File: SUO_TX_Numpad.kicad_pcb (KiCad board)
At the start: 2 copper layers, 79.1 x 127.6 mm, 94 parts, among them J1 USB_C_Receptacle_USB2.0_16P, SW1 BOOT, U1 STM32F411CEUx, U2 XC6206PxxxMR-Regulator_Linear, U3 USBLC6-2SC6

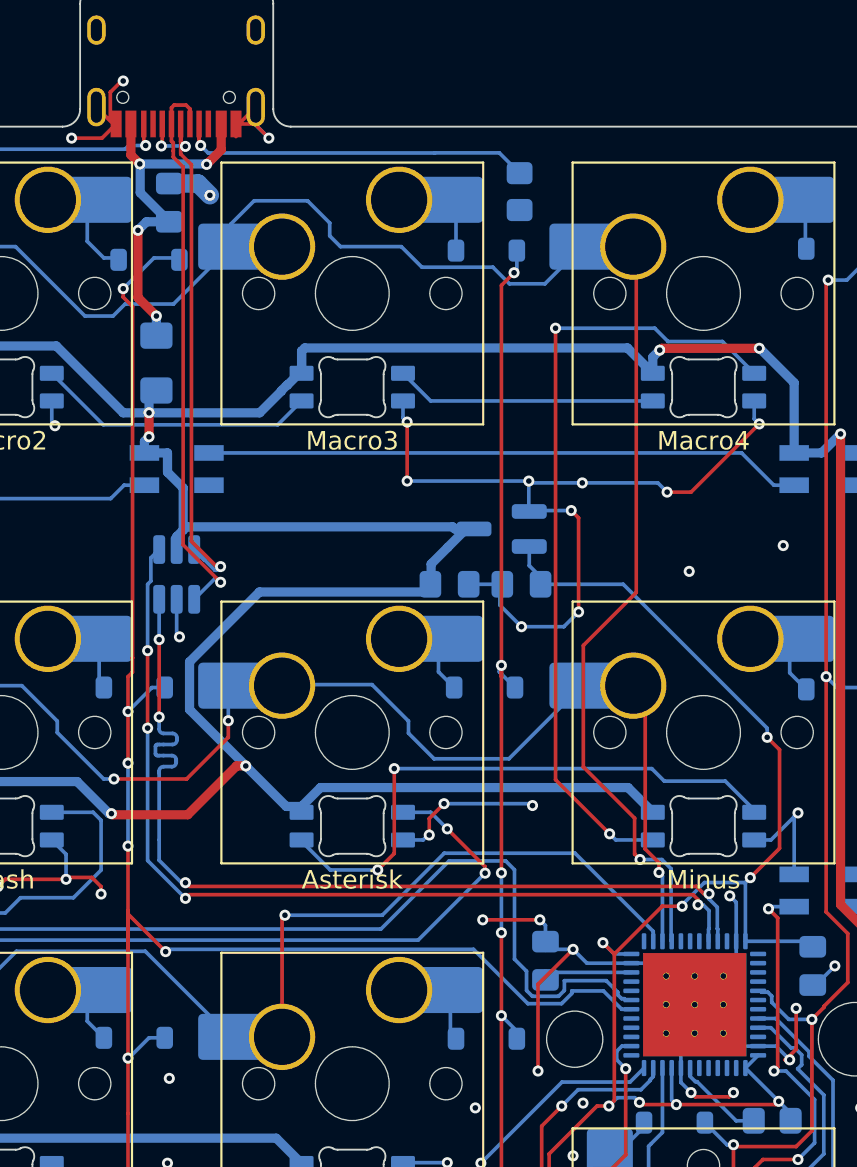
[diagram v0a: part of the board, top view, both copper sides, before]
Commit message: Updated BOM
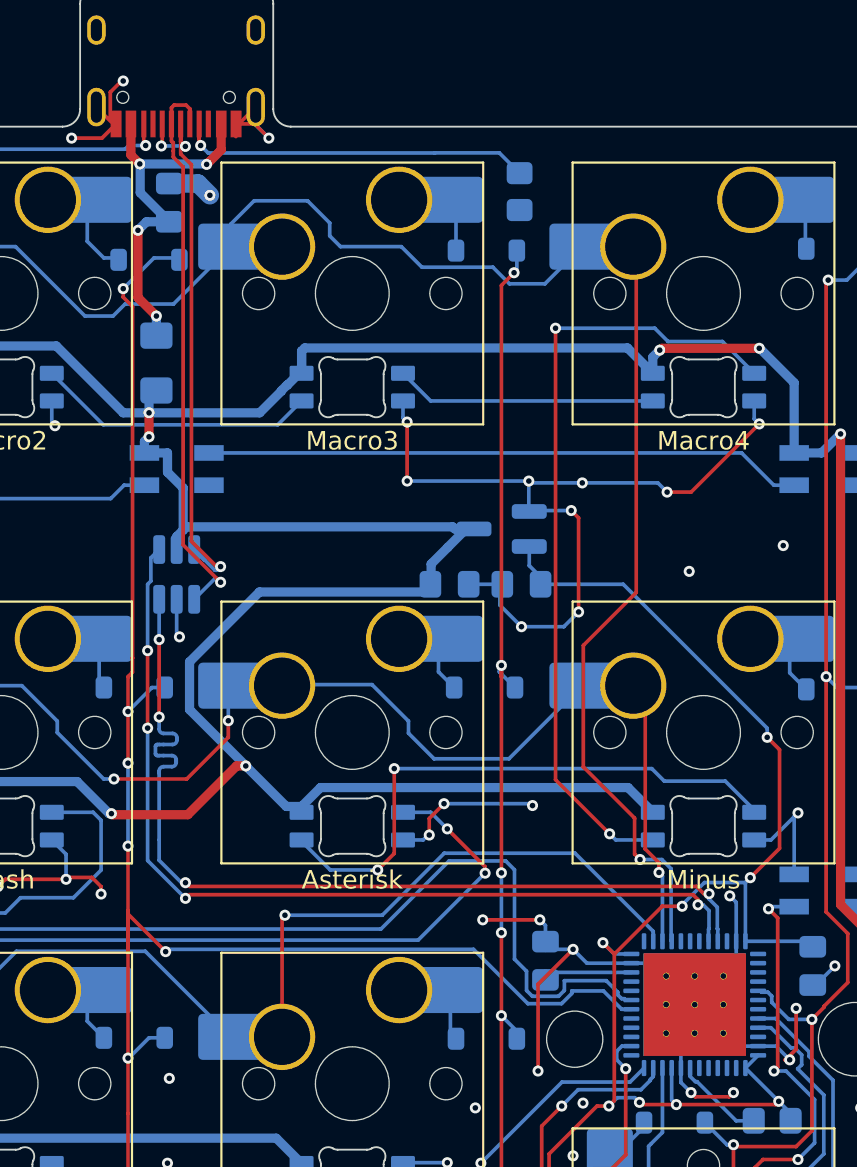
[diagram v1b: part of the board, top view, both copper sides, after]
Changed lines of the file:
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@@
 		)
 		(pad "A1" smd rect
-			(at -3.25 -4.045 180)
-			(size 0.6 1.45)
+			(at -3.255 -4.045 180)
+			(size 0.59 1.45)
 			(layers "F.Cu" "F.Mask" "F.Paste")
 			(net 14 "GND")
@@
 		(pad "A4" smd rect
 			(at -2.45 -4.045 180)
-			(size 0.6 1.45)
+			(size 0.58 1.45)
 			(layers "F.Cu" "F.Mask" "F.Paste")
 			(net 19 "USB_5V")
@@
 		(pad "A5" smd rect
 			(at -1.25 -4.045 180)
-			(size 0.3 1.45)
+			(size 0.28 1.45)
 			(layers "F.Cu" "F.Mask" "F.Paste")
 			(net 20 "Net-(J1-CC1)")
@@
 		(pad "A6" smd rect
 			(at -0.25 -4.045 180)
-			(size 0.3 1.45)
+			(size 0.28 1.45)
 			(layers "F.Cu" "F.Mask" "F.Paste")
 			(net 21 "USB_D+")
@@
 		(pad "A7" smd rect
 			(at 0.25 -4.045 180)
-			(size 0.3 1.45)
+			(size 0.28 1.45)
 			(layers "F.Cu" "F.Mask" "F.Paste")
 			(net 22 "USB_D-")
@@
 		(pad "A8" smd rect
 			(at 1.25 -4.045 180)
-			(size 0.3 1.45)
+			(size 0.28 1.45)
 			(layers "F.Cu" "F.Mask" "F.Paste")
 			(net 23 "unconnected-(J1-SBU1-PadA8)")
@@
 		(pad "A9" smd rect
 			(at 2.45 -4.045 180)
-			(size 0.6 1.45)
+			(size 0.58 1.45)
 			(layers "F.Cu" "F.Mask" "F.Paste")
 			(net 19 "USB_5V")
@@
 		)
 		(pad "A12" smd rect
-			(at 3.25 -4.045 180)
-			(size 0.6 1.45)
+			(at 3.255 -4.045 180)
+			(size 0.59 1.45)
 			(layers "F.Cu" "F.Mask" "F.Paste")
 			(net 14 "GND")
@@
 		)
 		(pad "B1" smd rect
-			(at 3.25 -4.045 180)
-			(size 0.6 1.45)
+			(at 3.255 -4.045 180)
+			(size 0.59 1.45)
 			(layers "F.Cu" "F.Mask" "F.Paste")
 			(net 14 "GND")
@@
 		(pad "B4" smd rect
 			(at 2.45 -4.045 180)
-			(size 0.6 1.45)
+			(size 0.58 1.45)
 			(layers "F.Cu" "F.Mask" "F.Paste")
 			(net 19 "USB_5V")
@@
 		(pad "B5" smd rect
 			(at 1.75 -4.045 180)
-			(size 0.3 1.45)
+			(size 0.28 1.45)
 			(layers "F.Cu" "F.Mask" "F.Paste")
 			(net 24 "Net-(J1-CC2)")
@@
 		(pad "B6" smd rect
 			(at 0.75 -4.045 180)
-			(size 0.3 1.45)
+			(size 0.28 1.45)
 			(layers "F.Cu" "F.Mask" "F.Paste")
 			(net 21 "USB_D+")
@@
 		(pad "B7" smd rect
 			(at -0.75 -4.045 180)
-			(size 0.3 1.45)
+			(size 0.28 1.45)
 			(layers "F.Cu" "F.Mask" "F.Paste")
 			(net 22 "USB_D-")
@@
 		(pad "B8" smd rect
 			(at -1.75 -4.045 180)
-			(size 0.3 1.45)
+			(size 0.28 1.45)
 			(layers "F.Cu" "F.Mask" "F.Paste")
 			(net 25 "unconnected-(J1-SBU2-PadB8)")
@@
 		(pad "B9" smd rect
 			(at -2.45 -4.045 180)
-			(size 0.6 1.45)
+			(size 0.58 1.45)
 			(layers "F.Cu" "F.Mask" "F.Paste")
 			(net 19 "USB_5V")
@@
 		)
 		(pad "B12" smd rect
-			(at -3.25 -4.045 180)
-			(size 0.6 1.45)
+			(at -3.255 -4.045 180)
+			(size 0.59 1.45)
 			(layers "F.Cu" "F.Mask" "F.Paste")
 			(net 14 "GND")
@@
 			)
 		)
-		(property "LCSC" "C60490"
+		(property "LCSC" "C2930231"
 			(at 0 0 0)
 			(unlocked yes)
@@
 			)
 		)
-		(property "LCSC" "C32949"
+		(property "LCSC" "C5137467"
 			(at 0 0 90)
 			(unlocked yes)
@@
 			)
 		)
-		(property "LCSC" "C315248"
+		(property "LCSC" "C49010152"
 			(at 0 0 0)
 			(unlocked yes)
@@
 			)
 		)
-		(property "LCSC" "C315248"
+		(property "LCSC" "C49010152"
 			(at 0 0 90)
 			(unlocked yes)
@@
 			)
 		)
-		(property "LCSC" "C105872"
+		(property "LCSC" "C2930296"
 			(at 0 0 270)
 			(unlocked yes)
@@
 			)
 		)
-		(property "LCSC" "C315248"
+		(property "LCSC" "C49010152"
 			(at 0 0 180)
 			(unlocked yes)
@@
 		(pad "49" smd rect
 			(at 0 0 90)
-			(size 5.6 5.6)
+			(size 5.56 5.56)
 			(property pad_prop_heatsink)
 			(layers "F.Cu")
@@
 		(pad "49" smd rect
 			(at 0 0 90)
-			(size 5.6 5.6)
+			(size 5.56 5.56)
 			(property pad_prop_heatsink)
 			(layers "B.Cu" "B.Mask")
@@
 			)
 		)
-		(property "LCSC" "C315248"
+		(property "LCSC" "C49010152"
 			(at 0 0 90)
 			(unlocked yes)
@@
 			)
 		)
-		(property "LCSC" "C60490"
+		(property "LCSC" "C2930231"
 			(at 0 0 180)
 			(unlocked yes)
@@
 			)
 		)
-		(property "LCSC" "C105872"
+		(property "LCSC" "C2930296"
 			(at 0 0 270)
 			(unlocked yes)
